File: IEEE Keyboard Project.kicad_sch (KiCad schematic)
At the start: 122 parts, among them U1 RP2354B

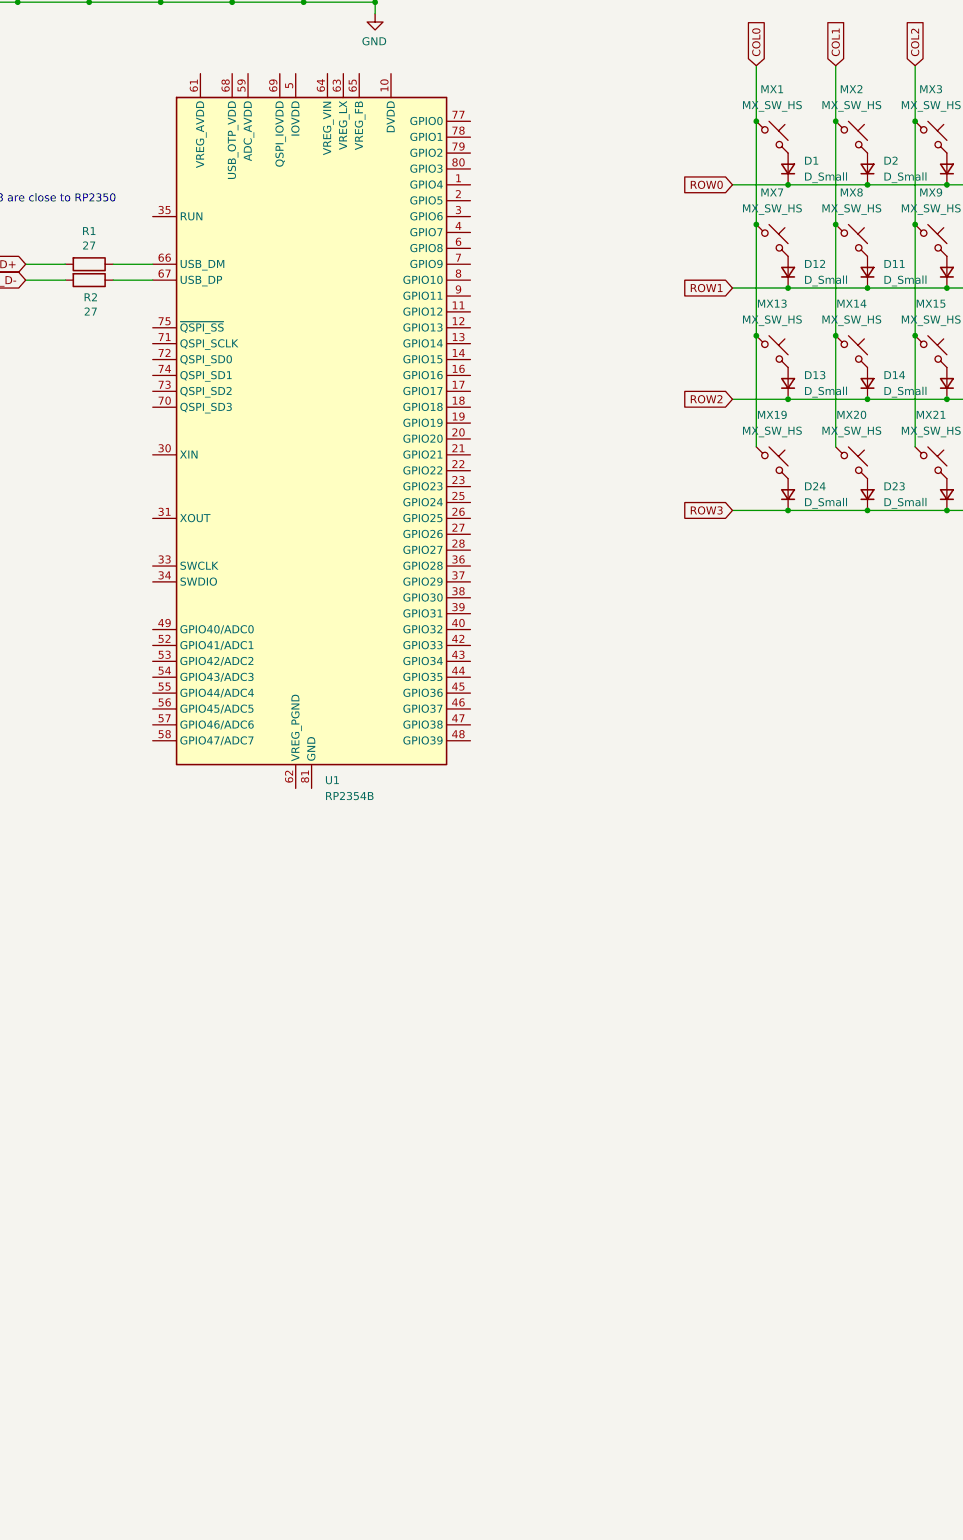
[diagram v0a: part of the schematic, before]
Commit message: Add files via upload
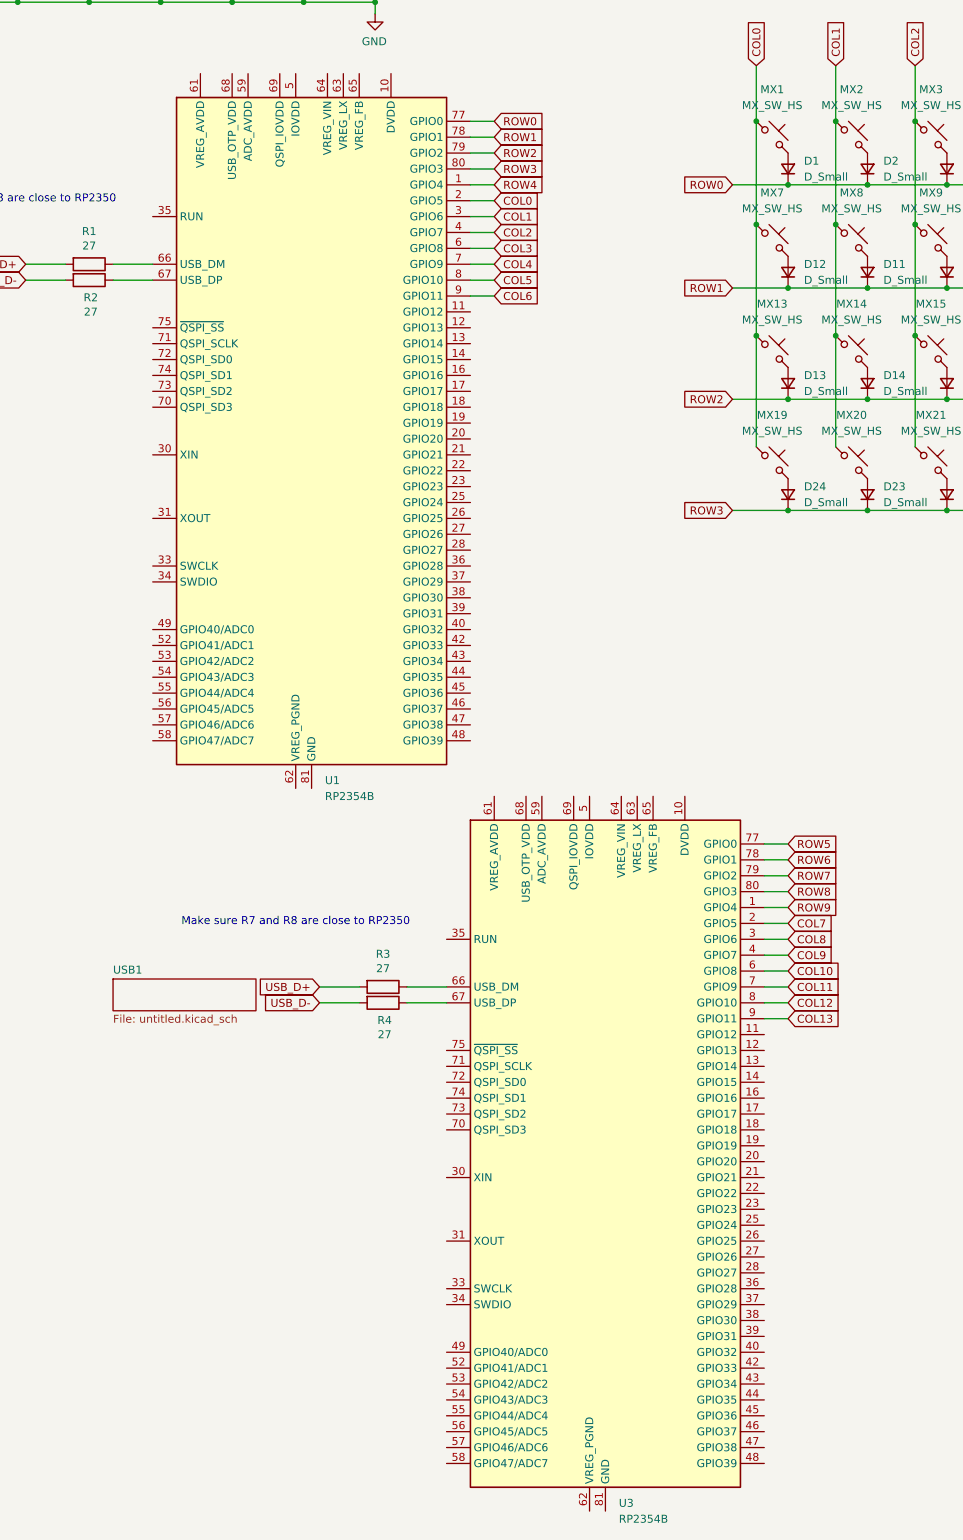
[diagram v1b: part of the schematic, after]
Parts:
- added R3, R4: 27, Resistor_SMD:R_0402_1005Metric, symbol Device:R
- added U3: RP2354B, Package_DFN_QFN:QFN-80-1EP_10x10mm_P0.4mm_EP3.4x3.4mm, symbol MCU_RaspberryPi:RP2354B
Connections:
- net COL0: now also U1.2 (GPIO5)
- net COL1: now also U1.3 (GPIO6)
- net COL10: now also U3.6 (GPIO8)
- net COL11: now also U3.7 (GPIO9)
- net COL12: now also U3.8 (GPIO10)
- net COL13: now also U3.9 (GPIO11)
- net COL2: now also U1.4 (GPIO7)
- net COL3: now also U1.6 (GPIO8)
- net COL4: now also U1.7 (GPIO9)
- net COL5: now also U1.8 (GPIO10)
- net COL6: now also U1.9 (GPIO11)
- net COL7: now also U3.2 (GPIO5)
- net COL8: now also U3.3 (GPIO6)
- net COL9: now also U3.4 (GPIO7)
- net ROW0: now also U1.77 (GPIO0)
- net ROW1: now also U1.78 (GPIO1)
- net ROW2: now also U1.79 (GPIO2)
- net ROW3: now also U1.80 (GPIO3)
- net ROW4: now also U1.1 (GPIO4)
- net ROW5: now also U3.77 (GPIO0)
- net ROW6: now also U3.78 (GPIO1)
- net ROW7: now also U3.79 (GPIO2)
- net ROW8: now also U3.80 (GPIO3)
- net ROW9: now also U3.1 (GPIO4)
- net USB_D+: now also R3.2
- net USB_D-: now also R4.2
- new net: R3.1, U3.66 (USB_DM)
- new net: U3.10 (DVDD), U3.32 (DVDD), U3.51 (DVDD)
- new net: U3.15 (IOVDD), U3.24 (IOVDD), U3.29 (IOVDD), U3.41 (IOVDD), U3.5 (IOVDD), U3.50 (IOVDD), U3.60 (IOVDD), U3.76 (IOVDD)
- new net: R4.1, U3.67 (USB_DP)
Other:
- added sheet USB1 (untitled.kicad_sch)

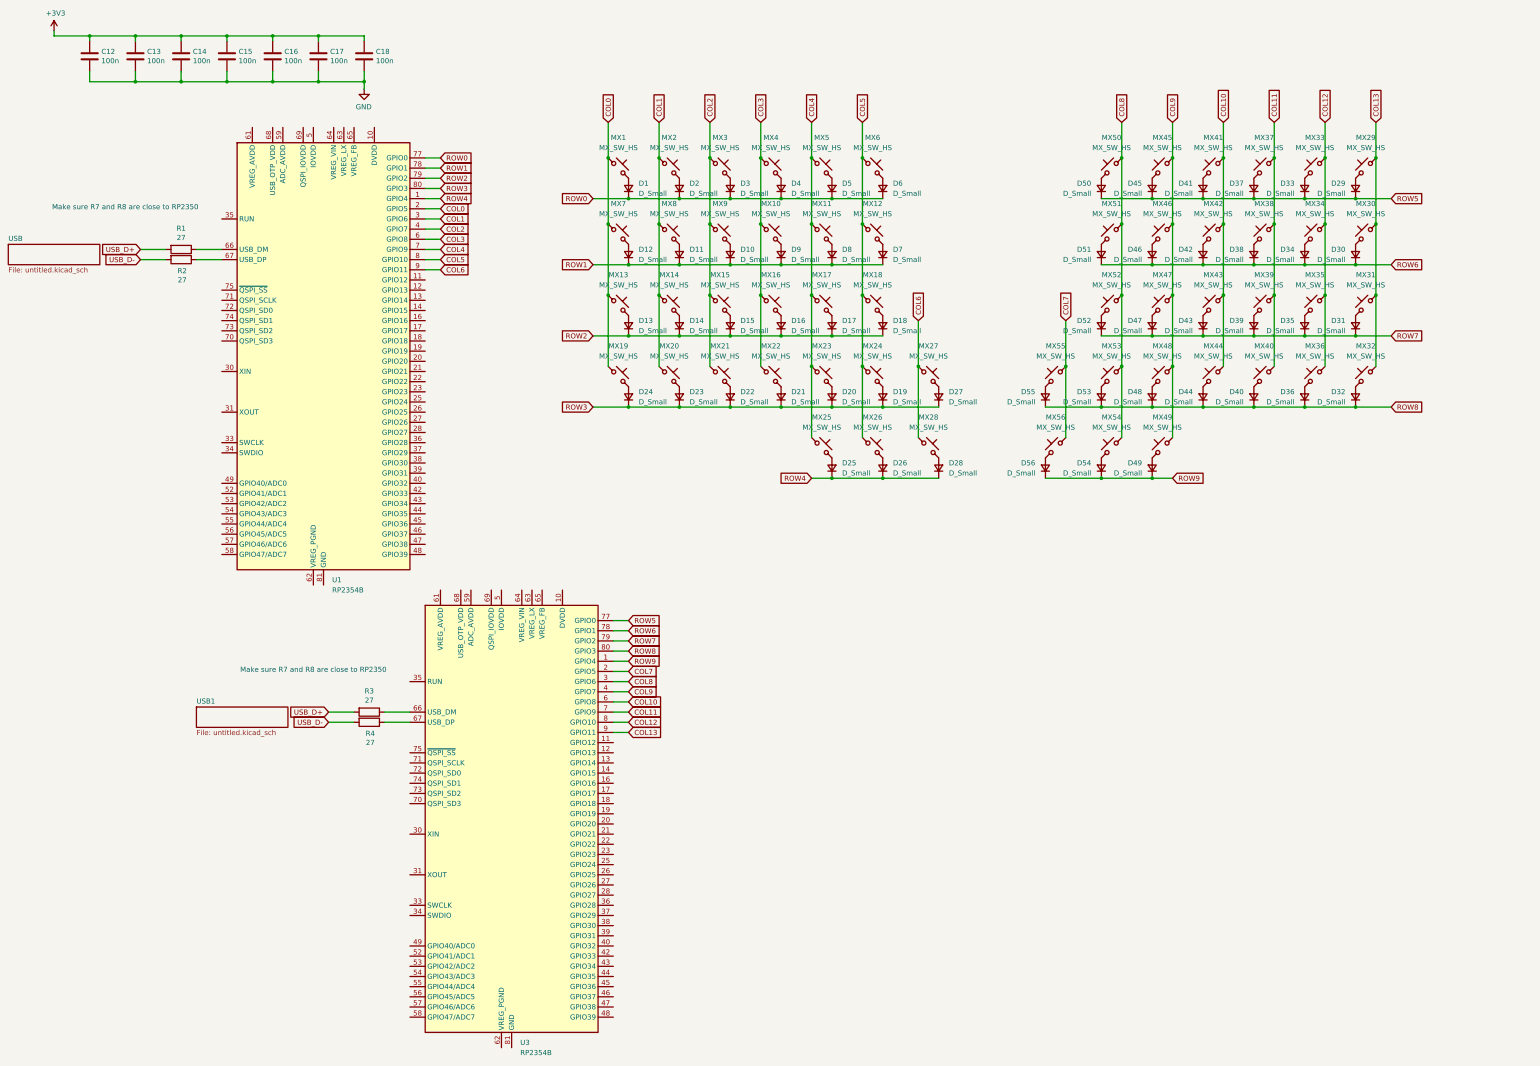
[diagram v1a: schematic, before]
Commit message: Add files via upload
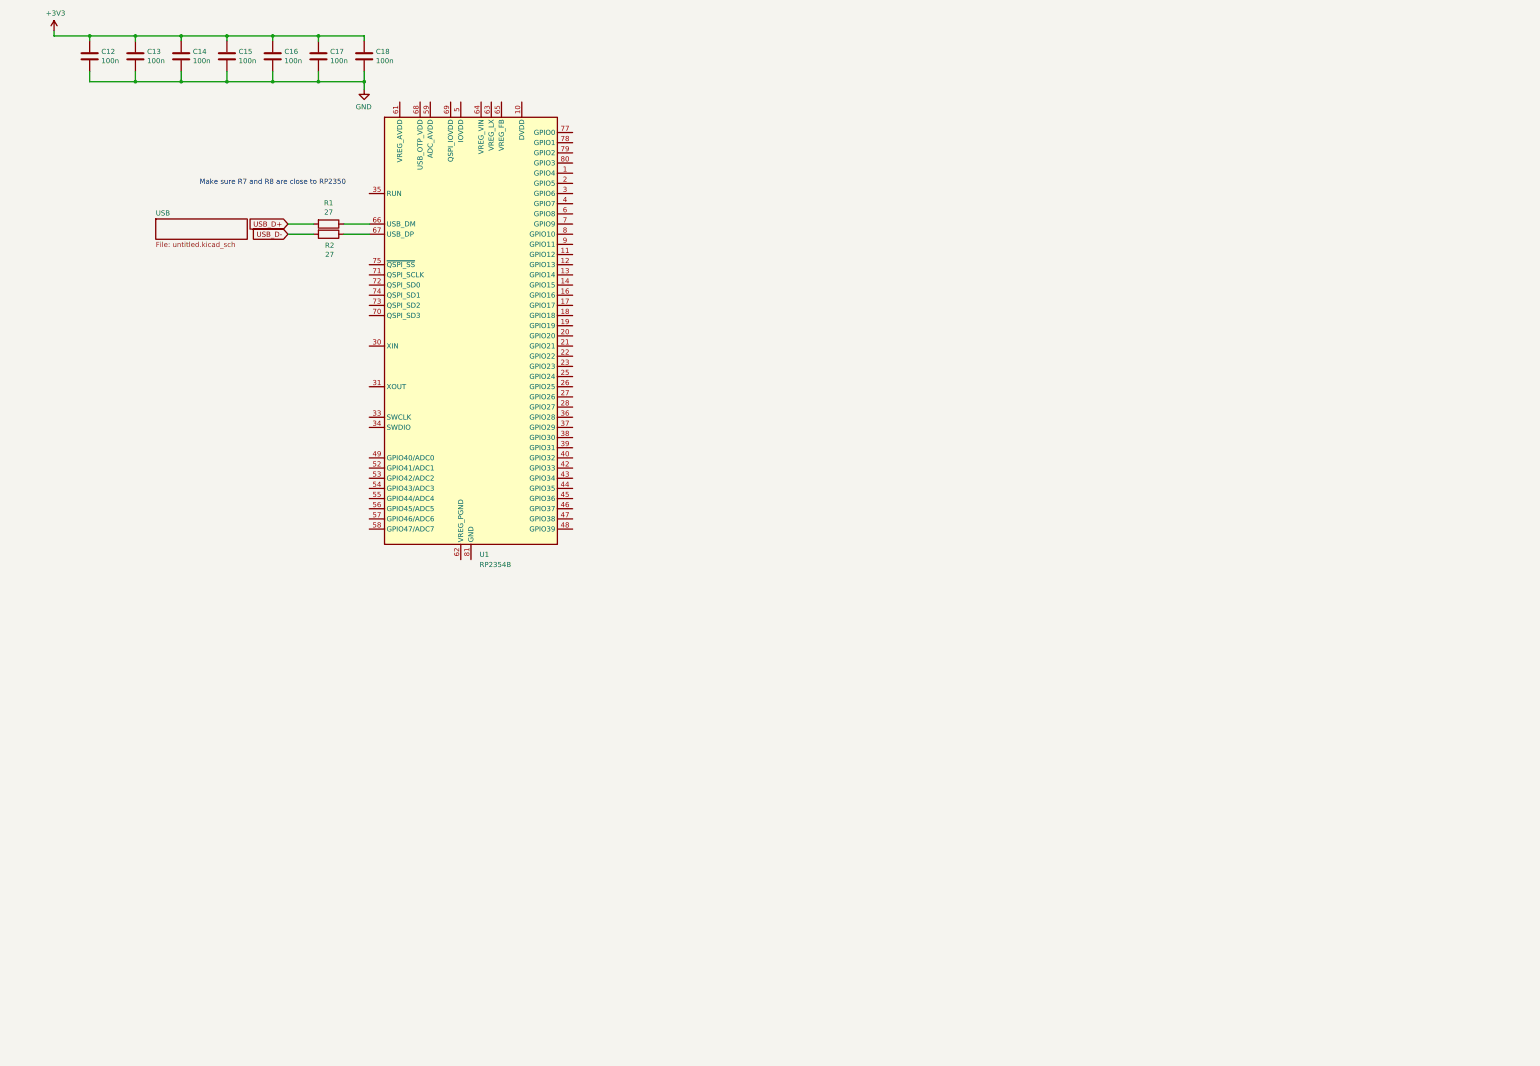
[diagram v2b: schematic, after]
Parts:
- removed D1, D10, D11, D12, D13, D14, D15, D16, D17, D18, D19, D2, D20, D21, D22, D23, D24, D25, D26, D27, D28, D29, D3, D30, D31, D32, D33, D34, D35, D36, D37, D38, D39, D4, D40, D41, D42, D43, D44, D45, D46, D47, D48, D49, D5, D50, D51, D52, D53, D54, D55, D56, D6, D7, D8, D9: D_Small, symbol Device:D_Small
- removed MX1, MX10, MX11, MX12, MX13, MX14, MX15, MX16, MX17, MX18, MX19, MX2, MX20, MX21, MX22, MX23, MX24, MX25, MX26, MX27, MX28, MX29, MX3, MX30, MX31, MX32, MX33, MX34, MX35, MX36, MX37, MX38, MX39, MX4, MX40, MX41, MX42, MX43, MX44, MX45, MX46, MX47, MX48, MX49, MX5, MX50, MX51, MX52, MX53, MX54, MX55, MX56, MX6, MX7, MX8, MX9: MX_SW_HS, Button_Switch_Keyboard:SW_Cherry_MX_1.00u_PCB, symbol marbastlib-mx:MX_SW_HS_CPG151101S11
- removed R3, R4: 27, Resistor_SMD:R_0402_1005Metric, symbol Device:R
- removed U3: RP2354B, Package_DFN_QFN:QFN-80-1EP_10x10mm_P0.4mm_EP3.4x3.4mm, symbol MCU_RaspberryPi:RP2354B
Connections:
- net COL0: no longer names the net of U1.2 (GPIO5)
- net COL1: no longer names the net of U1.3 (GPIO6)
- net COL2: no longer names the net of U1.4 (GPIO7)
- net COL3: no longer names the net of U1.6 (GPIO8)
- net COL4: no longer names the net of U1.7 (GPIO9)
- net COL5: no longer names the net of U1.8 (GPIO10)
- net COL6: no longer names the net of U1.9 (GPIO11)
- net ROW0: no longer names the net of U1.77 (GPIO0)
- net ROW1: no longer names the net of U1.78 (GPIO1)
- net ROW2: no longer names the net of U1.79 (GPIO2)
- net ROW3: no longer names the net of U1.80 (GPIO3)
- net ROW4: no longer names the net of U1.1 (GPIO4)
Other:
- removed sheet USB1
- moved on the sheet: R1, R2, U1

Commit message: Add files via upload
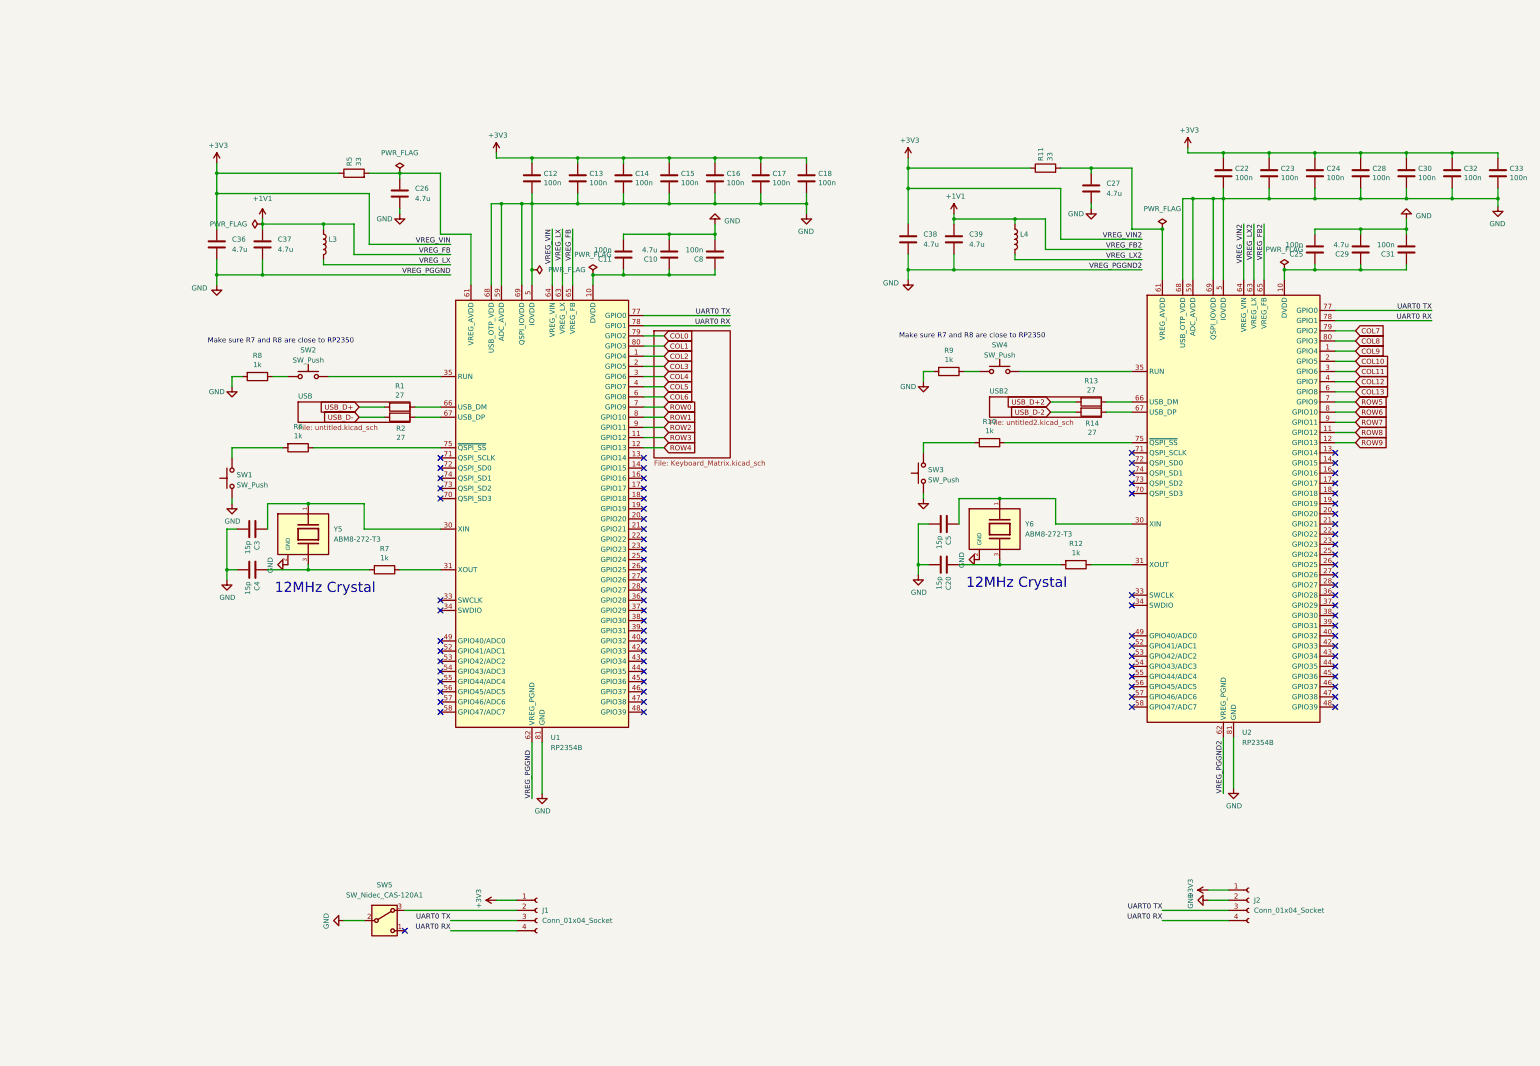
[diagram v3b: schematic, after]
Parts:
- added C10, C26, C27, C29, C36, C37, C38, C39: 4.7u, Capacitor_SMD:C_0402_1005Metric, symbol Device:C
- added C11, C22, C23, C24, C25, C28, C30, C31, C32, C33, C8: 100n, Capacitor_SMD:C_0402_1005Metric, symbol Device:C
- added C20, C3, C4, C5: 15p, Capacitor_SMD:C_0402_1005Metric, symbol Device:C
- added J1, J2: Conn_01x04_Socket, Connector_JST:JST_EH_S4B-EH_1x04_P2.50mm_Horizontal, symbol Connector:Conn_01x04_Socket
- added L3, L4: 3.3u, Inductor_SMD:L_Coilcraft_LPS3314, symbol Device:L
- added R10, R12, R6, R7, R8, R9: 1k, Resistor_SMD:R_0402_1005Metric, symbol Device:R
- added R11, R5: 33, Resistor_SMD:R_0402_1005Metric, symbol Device:R
- added R13, R14: 27, Resistor_SMD:R_0402_1005Metric, symbol Device:R
- added SW1, SW2, SW3, SW4: SW_Push, Button_Switch_SMD:SW_Push_1P1T_NO_Vertical_Wuerth_434133025816, symbol Switch:SW_Push
- added SW5: SW_Nidec_CAS-120A1, Button_Switch_SMD:Nidec_Copal_CAS-120A, symbol Switch:SW_Nidec_CAS-120A1
- added U2: RP2354B, Package_DFN_QFN:QFN-80-1EP_10x10mm_P0.4mm_EP3.4x3.4mm, symbol MCU_RaspberryPi:RP2354B
- added Y5, Y6: ABM8-272-T3, ABM8-272-T3:XTAL_ABM8-272-T3, symbol ABM8-272-T3:ABM8-272-T3
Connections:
- net +3V3: now also U1.64 (VREG_VIN), C22.1, C23.1, C24.1, C28.1, C30.1, C32.1, C33.1, C36.1, C38.1, J1.1 (Pin_1), J2.1 (Pin_1), R11.1, R5.1, U2.64 (VREG_VIN)
- net GND: now also U1.15 (IOVDD), U1.24 (IOVDD), U1.29 (IOVDD), U1.41 (IOVDD), U1.5 (IOVDD), U1.50 (IOVDD), U1.59 (ADC_AVDD), U1.60 (IOVDD), U1.62 (VREG_PGND), U1.68 (USB_OTP_VDD), U1.69 (QSPI_IOVDD), U1.76 (IOVDD), U1.81 (GND), C10.2, C11.2, C20.2, C22.2, C23.2, C24.2, C25.2, C26.2, C27.2, C28.2, C29.2, C3.2, C30.2, C31.2, C32.2, C33.2, C36.2, C37.2, C38.2, C39.2, C4.2, C5.2, C8.2, J2.2 (Pin_2), R8.2, R9.2, SW1.1, SW3.1, SW5.2 (B), U2.15 (IOVDD), U2.24 (IOVDD), U2.29 (IOVDD), U2.41 (IOVDD), U2.5 (IOVDD), U2.50 (IOVDD), U2.59 (ADC_AVDD), U2.60 (IOVDD), U2.62 (VREG_PGND), U2.68 (USB_OTP_VDD), U2.69 (QSPI_IOVDD), U2.76 (IOVDD), U2.81 (GND), Y5.2 (GND), Y5.4 (GND), Y6.2 (GND), Y6.4 (GND)
- net COL2: now reaches U1.1 (GPIO4)
- net at U1.10 (DVDD), U1.32 (DVDD), U1.51 (DVDD): now also C10.1, C11.1, C8.1
- net ROW3: now reaches U1.11 (GPIO12)
- net ROW4: now reaches U1.12 (GPIO13)
- net COL3: now reaches U1.2 (GPIO5)
- net COL4: now reaches U1.3 (GPIO6)
- net at U1.30 (XIN): now also C3.1, Y5.1
- net at U1.31 (XOUT): now also R7.1
- net at U1.35 (RUN): now also SW2.2
- net COL5: now reaches U1.4 (GPIO7)
- net COL6: now reaches U1.6 (GPIO8)
- net at U1.61 (VREG_AVDD): now also C26.1, R5.2
- net VREG_LX: now reaches U1.63 (VREG_LX)
- net VREG_LX: now also L3.2
- net +1V1: now reaches U1.65 (VREG_FB)
- net +1V1: now also C37.1, C39.1, L3.1, L4.1, U2.65 (VREG_FB)
- net ROW0: now reaches U1.7 (GPIO9)
- net at U1.75 (~{QSPI_SS}): now also R6.1
- net UART0 TX: now reaches U1.77 (GPIO0)
- net UART0 TX: now also J1.3 (Pin_3), J2.3 (Pin_3), U2.77 (GPIO0)
- net UART0 RX: now reaches U1.78 (GPIO1)
- net UART0 RX: now also J1.4 (Pin_4), J2.4 (Pin_4), U2.78 (GPIO1)
- net COL0: now reaches U1.79 (GPIO2)
- net ROW1: now reaches U1.8 (GPIO10)
- net COL1: now reaches U1.80 (GPIO3)
- net ROW2: now reaches U1.9 (GPIO11)
- new net: R12.1, U2.31 (XOUT)
- new net: C20.1, R12.2, Y6.3
- new net: C25.1, C29.1, C31.1, U2.10 (DVDD), U2.32 (DVDD), U2.51 (DVDD)
- new net: R9.1, SW4.1
- new net: SW4.2, U2.35 (RUN)
- new net: R10.1, U2.75 (~{QSPI_SS})
- new net: R10.2, SW3.2
- new net: C5.1, U2.30 (XIN), Y6.1
- new net: R8.1, SW2.1
- new net: C4.1, R7.2, Y5.3
- new net: R6.2, SW1.2
- new net: C27.1, R11.2, U2.61 (VREG_AVDD)
- new net: R13.1, U2.66 (USB_DM)
- new net: R14.1, U2.67 (USB_DP)
- new net: J1.2 (Pin_2), SW5.3 (A)
- new net COL10: U2.2 (GPIO5)
- new net COL11: U2.3 (GPIO6)
- new net COL12: U2.4 (GPIO7)
- new net COL13: U2.6 (GPIO8)
- new net COL7: U2.79 (GPIO2)
- new net COL8: U2.80 (GPIO3)
- new net COL9: U2.1 (GPIO4)
- new net ROW5: U2.7 (GPIO9)
- new net ROW6: U2.8 (GPIO10)
- new net ROW7: U2.9 (GPIO11)
- new net ROW8: U2.11 (GPIO12)
- new net ROW9: U2.12 (GPIO13)
- new net USB_D+2: R13.2
- new net USB_D-2: R14.2
- new net VREG_LX2: L4.2, U2.63 (VREG_LX)
- no-connect marks 0 -> 83
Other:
- added sheet Keyboard Matrix (Keyboard_Matrix.kicad_sch)
- added sheet USB2 (untitled2.kicad_sch)
- note added: "12MHz Crystal"
- moved on the sheet: C12, C13, C14, C15, C16, C17, C18, R1, R2, U1
